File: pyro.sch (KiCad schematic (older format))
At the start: 10 parts, among them J10 Screw_Terminal_01x02, J9 Screw_Terminal_01x02, Q2 PMV20ENR, U10 LTV-817S

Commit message: Cleaned up layout, added barrel jack for power input
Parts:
- JP1: footprint Jumper:SolderJumper-3_P2.0mm_Open_TrianglePad1.0x1.5mm -> Jumper:SolderJumper-3_P1.3mm_Open_RoundedPad1.0x1.5mm_NumberLabels
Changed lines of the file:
@@
 F 0 "JP1" H 4450 2855 50  0000 C CNN
 F 1 "SolderJumper_3_Open" H 4450 2764 50  0000 C CNN
-F 2 "Jumper:SolderJumper-3_P2.0mm_Open_TrianglePad1.0x1.5mm" H 4450 2650 50  0001 C CNN
+F 2 "Jumper:SolderJumper-3_P1.3mm_Open_RoundedPad1.0x1.5mm_NumberLabels" H 4450 2650 50  0001 C CNN
 F 3 "~" H 4450 2650 50  0001 C CNN
 	1    4450 2650

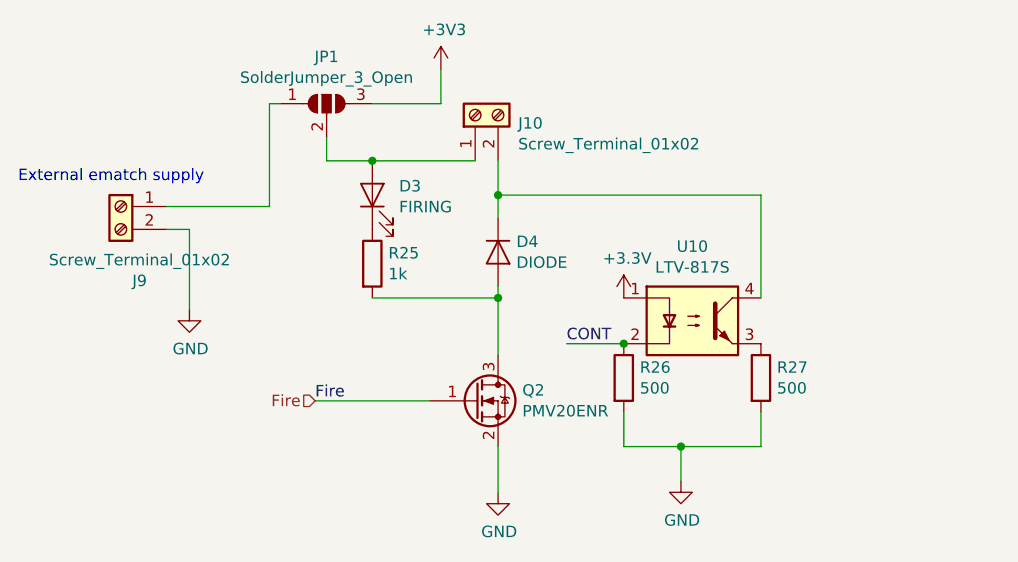
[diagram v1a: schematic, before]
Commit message: Added 3D models, added ptaps sheet, fixed pyros
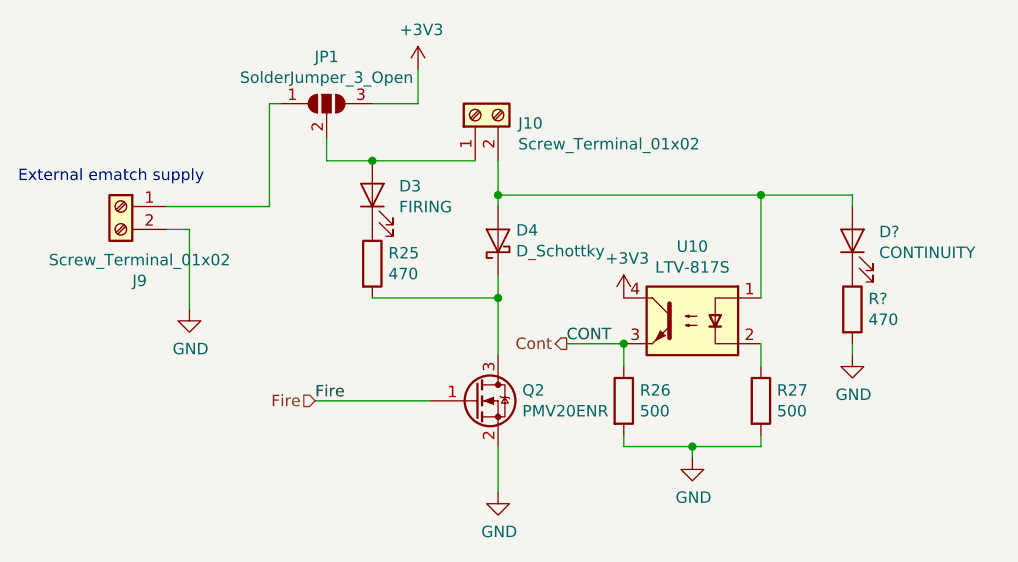
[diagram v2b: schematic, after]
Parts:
- removed D4: DIODE, Diode_SMD:D_SMA, symbol Device:D
- added D4: D_Schottky, Diode_SMD:D_SOD-123F, symbol Device:D_Schottky
- added D?: CONTINUITY, LED_SMD:LED_0805_2012Metric, symbol Device:LED
- added R?: 470, Resistor_SMD:R_0603_1608Metric, symbol Device:R
- R25: value 1k -> 470
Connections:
- net +3V3: now also U10.4; no longer U10.1
- net GND: now also R?.2
- net at J10.2 (Pin_2): now also U10.1, D4.2 (A), D?.2 (A); no longer U10.4
- net at Q2.3 (D), R25.2: now also D4.1 (K)
- net at R27.1: now also U10.2; no longer U10.3
- net CONT renamed Cont
- net Cont: now also U10.3; no longer U10.2
- new net: D?.1 (K), R?.1
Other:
- moved on the sheet: R26, R27
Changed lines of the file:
@@
 $Descr A4 11693 8268
 encoding utf-8
-Sheet 4 5
+Sheet 4 6
 Title ""
 Date ""
@@
 P 4650 3350
 F 0 "R25" H 4720 3396 50  0000 L CNN
-F 1 "1k" H 4720 3305 50  0000 L CNN
+F 1 "470" H 4720 3305 50  0000 L CNN
 F 2 "Resistor_SMD:R_0603_1608Metric" V 4580 3350 50  0001 C CNN
 F 3 "~" H 4650 3350 50  0001 C CNN
@@
 Wire Wire Line
 	4650 2900 5100 2900
-$Comp
-L Device:D D?
-U 1 1 5DBDF40B
-P 5200 3300
-AR Path="/5DBDF40B" Ref="D?"  Part="1"
-AR Path="/5DB4FA2A/5DBDF40B" Ref="D4"  Part="1"
-F 0 "D4" V 5154 3380 50  0000 L CNN
-F 1 "DIODE" V 5245 3380 50  0000 L CNN
-F 2 "Diode_SMD:D_SMA" H 5200 3300 50  0001 C CNN
-F 3 "~" H 5200 3300 50  0001 C CNN
-F 4 "Y" H 5200 3300 50  0001 L CNN "Spice_Netlist_Enabled"
-F 5 "V" H 5200 3300 50  0001 L CNN "Spice_Primitive"
-	1    5200 3300
-	0    1    1    0
-$EndComp
-Wire Wire Line
-	5200 3450 5200 3500
+Wire Wire Line
+	5200 3400 5200 3500
 Wire Wire Line
 	4650 3500 5200 3500
@@
 Connection ~ 5200 3050
 Wire Wire Line
-	5200 3050 5200 3150
+	5200 3050 5200 3100
 $Comp
 L Isolator:LTV-817S U10
@@
 F 3 "http://www.us.liteon.com/downloads/LTV-817-827-847.PDF" H 5700 3900 50  0001 C CNN
 	1    6050 3600
-	1    0    0    -1
+	-1   0    0    -1
 $EndComp
 Wire Wire Line
@@
 L Device:R R27
 U 1 1 5DBE9B58
-P 6350 3850
-F 0 "R27" H 6420 3896 50  0000 L CNN
-F 1 "500" H 6420 3805 50  0000 L CNN
-F 2 "Resistor_SMD:R_0603_1608Metric" V 6280 3850 50  0001 C CNN
-F 3 "~" H 6350 3850 50  0001 C CNN
-	1    6350 3850
-	1    0    0    -1
-$EndComp
-Wire Wire Line
-	6350 4000 6350 4150
-Wire Wire Line
-	6350 4150 6000 4150
-Wire Wire Line
-	6000 4150 6000 4300
+P 6350 3950
+F 0 "R27" H 6420 3996 50  0000 L CNN
+F 1 "500" H 6420 3905 50  0000 L CNN
+F 2 "Resistor_SMD:R_0603_1608Metric" V 6280 3950 50  0001 C CNN
+F 3 "~" H 6350 3950 50  0001 C CNN
+	1    6350 3950
+	1    0    0    -1
+$EndComp
+Wire Wire Line
+	6350 4150 6050 4150
+Wire Wire Line
+	6050 4150 6050 4200
 $Comp
 L power:GND #PWR055
 U 1 1 5DBEA959
-P 6000 4300
-F 0 "#PWR055" H 6000 4050 50  0001 C CNN
-F 1 "GND" H 6005 4127 50  0000 C CNN
-F 2 "" H 6000 4300 50  0001 C CNN
-F 3 "" H 6000 4300 50  0001 C CNN
-	1    6000 4300
-	1    0    0    -1
-$EndComp
-$Comp
-L power:+3.3V #PWR054
-U 1 1 5DBEE894
-P 5750 3500
-F 0 "#PWR054" H 5750 3350 50  0001 C CNN
-F 1 "+3.3V" H 5765 3673 50  0000 C CNN
-F 2 "" H 5750 3500 50  0001 C CNN
-F 3 "" H 5750 3500 50  0001 C CNN
-	1    5750 3500
+P 6050 4200
+F 0 "#PWR055" H 6050 3950 50  0001 C CNN
+F 1 "GND" H 6055 4027 50  0000 C CNN
+F 2 "" H 6050 4200 50  0001 C CNN
+F 3 "" H 6050 4200 50  0001 C CNN
+	1    6050 4200
 	1    0    0    -1
 $EndComp
@@
 L Device:R R26
 U 1 1 5DBEF42E
-P 5750 3850
-F 0 "R26" H 5820 3896 50  0000 L CNN
-F 1 "500" H 5820 3805 50  0000 L CNN
-F 2 "Resistor_SMD:R_0603_1608Metric" V 5680 3850 50  0001 C CNN
-F 3 "~" H 5750 3850 50  0001 C CNN
-	1    5750 3850
-	1    0    0    -1
-$EndComp
-Wire Wire Line
-	5750 4000 5750 4150
-Wire Wire Line
-	5750 4150 6000 4150
-Connection ~ 6000 4150
+P 5750 3950
+F 0 "R26" H 5820 3996 50  0000 L CNN
+F 1 "500" H 5820 3905 50  0000 L CNN
+F 2 "Resistor_SMD:R_0603_1608Metric" V 5680 3950 50  0001 C CNN
+F 3 "~" H 5750 3950 50  0001 C CNN
+	1    5750 3950
+	1    0    0    -1
+$EndComp
+Wire Wire Line
+	5750 4150 6050 4150
+Connection ~ 6050 4150
 Text Label 4400 3950 0    50   ~ 0
 Fire
 Wire Wire Line
 	5750 3700 5500 3700
-Connection ~ 5750 3700
 Text Label 5500 3700 0    50   ~ 0
 CONT
@@
 Wire Wire Line
 	4200 2650 4200 3100
-$Comp
-L power:+3V3 #PWR052
-U 1 1 5DB4F735
-P 4950 2500
-F 0 "#PWR052" H 4950 2350 50  0001 C CNN
-F 1 "+3V3" H 4965 2673 50  0000 C CNN
-F 2 "" H 4950 2500 50  0001 C CNN
-F 3 "" H 4950 2500 50  0001 C CNN
-	1    4950 2500
-	1    0    0    -1
-$EndComp
-Wire Wire Line
-	4650 2650 4950 2650
-Wire Wire Line
-	4950 2650 4950 2500
+Wire Wire Line
+	4650 2650 4850 2650
+Wire Wire Line
+	4850 2650 4850 2500
 Text Notes 3100 3000 0    50   ~ 0
 External ematch supply
 Text HLabel 4400 3950 0    50   Input ~ 0
 Fire
+$Comp
+L Device:D_Schottky D?
+U 1 1 5DCE52FA
+P 5200 3250
+AR Path="/5DAD2180/5DCE52FA" Ref="D?"  Part="1"
+AR Path="/5DB4FA2A/5DCE52FA" Ref="D4"  Part="1"
+F 0 "D4" V 5246 3171 50  0000 R CNN
+F 1 "D_Schottky" V 5155 3171 50  0000 R CNN
+F 2 "Diode_SMD:D_SOD-123F" H 5200 3250 50  0001 C CNN
+F 3 "http://www.smc-diodes.com/propdf/DSS12U%20THRU%20DSS125U%20N1873%20REV.A.pdf" H 5200 3250 50  0001 C CNN
+	1    5200 3250
+	0    -1   -1   0
+$EndComp
+Wire Wire Line
+	5750 4100 5750 4150
+Wire Wire Line
+	6350 4100 6350 4150
+Wire Wire Line
+	6350 3800 6350 3700
+Wire Wire Line
+	5750 3800 5750 3700
+Connection ~ 5750 3700
+Text HLabel 5500 3700 0    50   Output ~ 0
+Cont
+$Comp
+L Device:R R?
+U 1 1 5DD2B596
+P 6750 3550
+F 0 "R?" H 6820 3596 50  0000 L CNN
+F 1 "470" H 6820 3505 50  0000 L CNN
+F 2 "Resistor_SMD:R_0603_1608Metric" V 6680 3550 50  0001 C CNN
+F 3 "~" H 6750 3550 50  0001 C CNN
+	1    6750 3550
+	1    0    0    -1
+$EndComp
+$Comp
+L Device:LED D?
+U 1 1 5DD2B5A0
+P 6750 3250
+F 0 "D?" V 6789 3133 50  0000 R CNN
+F 1 "CONTINUITY" V 6698 3133 50  0000 R CNN
+F 2 "LED_SMD:LED_0805_2012Metric" H 6750 3250 50  0001 C CNN
+F 3 "~" H 6750 3250 50  0001 C CNN
+	1    6750 3250
+	0    -1   -1   0
+$EndComp
+Wire Wire Line
+	6350 3050 6750 3050
+Wire Wire Line
+	6750 3050 6750 3100
+Connection ~ 6350 3050
+$Comp
+L power:GND #PWR?
+U 1 1 5DD2EA4C
+P 6750 3750
+F 0 "#PWR?" H 6750 3500 50  0001 C CNN
+F 1 "GND" H 6755 3577 50  0000 C CNN
+F 2 "" H 6750 3750 50  0001 C CNN
+F 3 "" H 6750 3750 50  0001 C CNN
+	1    6750 3750
+	1    0    0    -1
+$EndComp
+Wire Wire Line
+	6750 3750 6750 3700
+$Comp
+L power:+3V3 #PWR052
+U 1 1 5DB4F735
+P 4850 2500
+F 0 "#PWR052" H 4850 2350 50  0001 C CNN
+F 1 "+3V3" H 4865 2673 50  0000 C CNN
+F 2 "" H 4850 2500 50  0001 C CNN
+F 3 "" H 4850 2500 50  0001 C CNN
+	1    4850 2500
+	1    0    0    -1
+$EndComp
+$Comp
+L power:+3V3 #PWR?
+U 1 1 5DD30CD3
+P 5750 3500
+F 0 "#PWR?" H 5750 3350 50  0001 C CNN
+F 1 "+3V3" H 5765 3673 50  0000 C CNN
+F 2 "" H 5750 3500 50  0001 C CNN
+F 3 "" H 5750 3500 50  0001 C CNN
+	1    5750 3500
+	1    0    0    -1
+$EndComp
 $EndSCHEMATC
